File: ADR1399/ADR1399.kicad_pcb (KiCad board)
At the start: 2 copper layers, 106.7 x 55.9 mm, 80 parts, among them J1 10V, J2 Conn_01x04_Male, J3 4V6, J4 7V, J5 Conn_01x02_Male, J6 Conn_01x02_Male, J7 Conn_01x01_Male, Q1 BC547, Q2 BC547, U1 OPA2182xD, U2 LM399, U3 OPA2186xD, U4 OPA2209xD, U5 LM7815_TO220

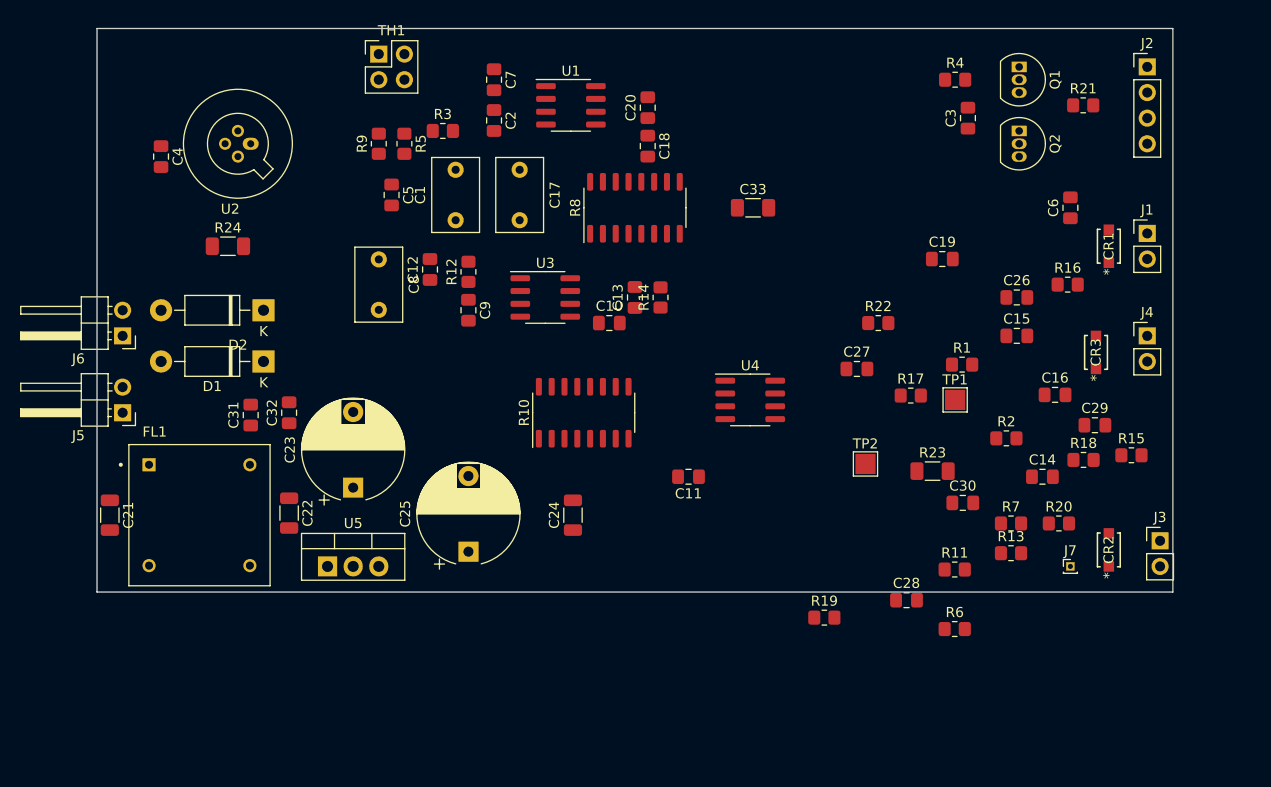
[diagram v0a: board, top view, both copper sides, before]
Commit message: Push the local work from Ryzen5600G PC part 1
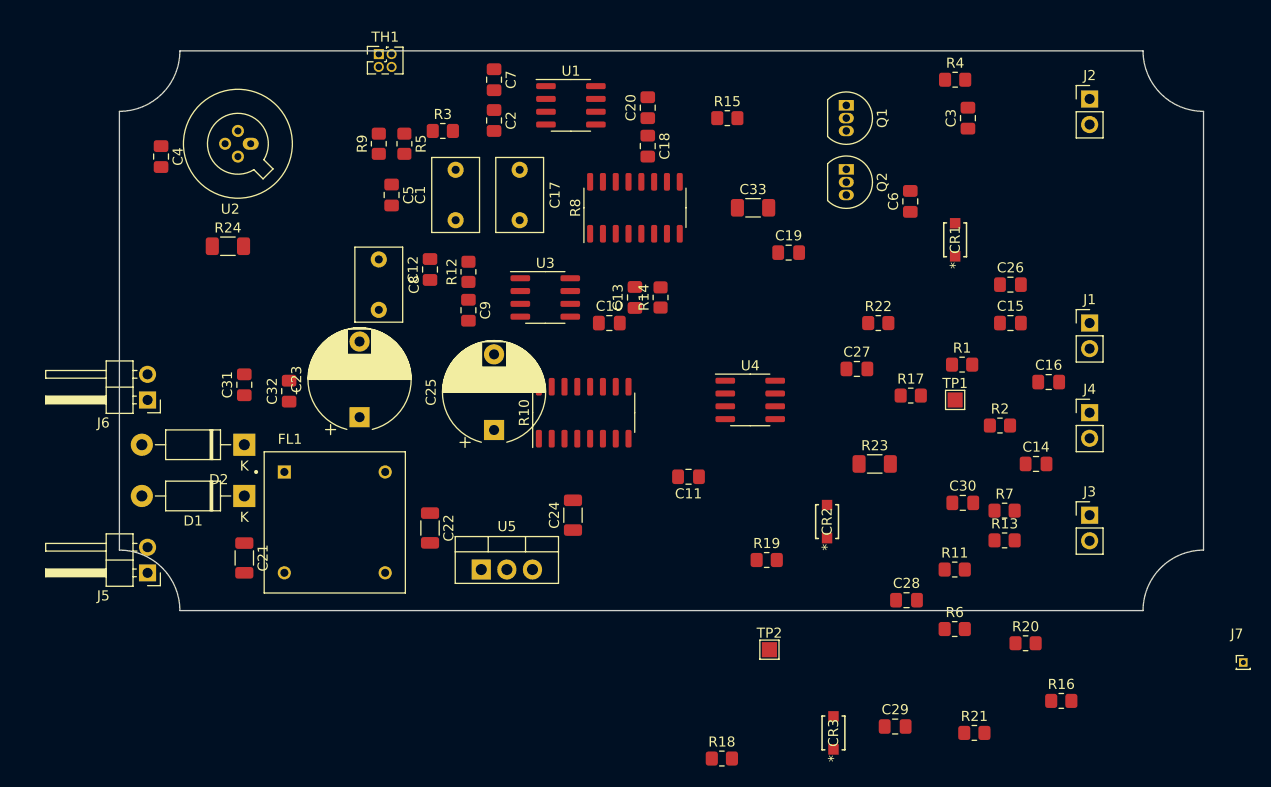
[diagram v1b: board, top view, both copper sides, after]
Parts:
- CR1: value SZSMF4L12AT3G -> SZSMF4L12AT3G
- CR2: value SZSMF4L6.5AT3G -> SZSMF4L6.5AT3G
- CR3: value SZSMF4L8.5AT3G -> SZSMF4L8.5AT3G
- J2: value Conn_01x04_Male -> PT100; footprint Connector_PinHeader_2.54mm:PinHeader_1x04_P2.54mm_Vertical -> Connector_PinHeader_2.54mm:PinHeader_1x02_P2.54mm_Vertical
- TH1: footprint Connector_PinHeader_2.54mm:PinHeader_2x02_P2.54mm_Vertical -> Connector_PinHeader_1.27mm:PinHeader_2x02_P1.27mm_Vertical
- TP1, TP2: value (none) -> ~; footprint TestPoint:TestPoint_Pad_2.0x2.0mm -> TestPoint:TestPoint_Pad_1.5x1.5mm
- moved R21 63.2 mm to (104.8, 87.6)
- moved R15 52.2 mm to (80.3, 26.7)
- moved R18 46.5 mm to (79.7, 90.2)
- moved CR3 45.8 mm to (90.8, 87.6)
- moved R16 41.3 mm to (113.4, 84.5)
- moved C29 35.8 mm to (96.9, 87.0)
- moved CR2 28.1 mm to (90.2, 66.7)
- moved TP2 20.7 mm to (84.5, 79.4)
- moved J7 19.6 mm to (131.4, 80.6)
- moved Q1 17.6 mm to (92.1, 25.4)
- moved Q2 17.6 mm to (92.1, 31.8)
- moved J5 16.1 mm to (22.8, 71.8)
- moved C6 15.9 mm to (98.4, 34.9)
- moved C19 15.3 mm to (86.4, 40.0)
- moved CR1 15.3 mm to (102.9, 38.7)
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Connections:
- J2 pad 1: Net-(J2-Pad1) -> Net-(J2-Pin_1)
- J2 pad 2: Net-(J2-Pad1) -> Net-(J2-Pin_2)
- TH1 pad 1: Net-(J2-Pad1) -> Net-(J2-Pin_2)
- TH1 pad 2: Net-(J2-Pad1) -> Net-(J2-Pin_2)
- TH1 pad 3: Net-(J2-Pad3) -> Net-(J2-Pin_1)
- TH1 pad 4: Net-(J2-Pad3) -> Net-(J2-Pin_1)
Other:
- board size 106.7 x 55.9 mm -> 107.5 x 55.5 mm
- copper layers 2 -> 4
